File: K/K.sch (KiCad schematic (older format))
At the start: 75 parts

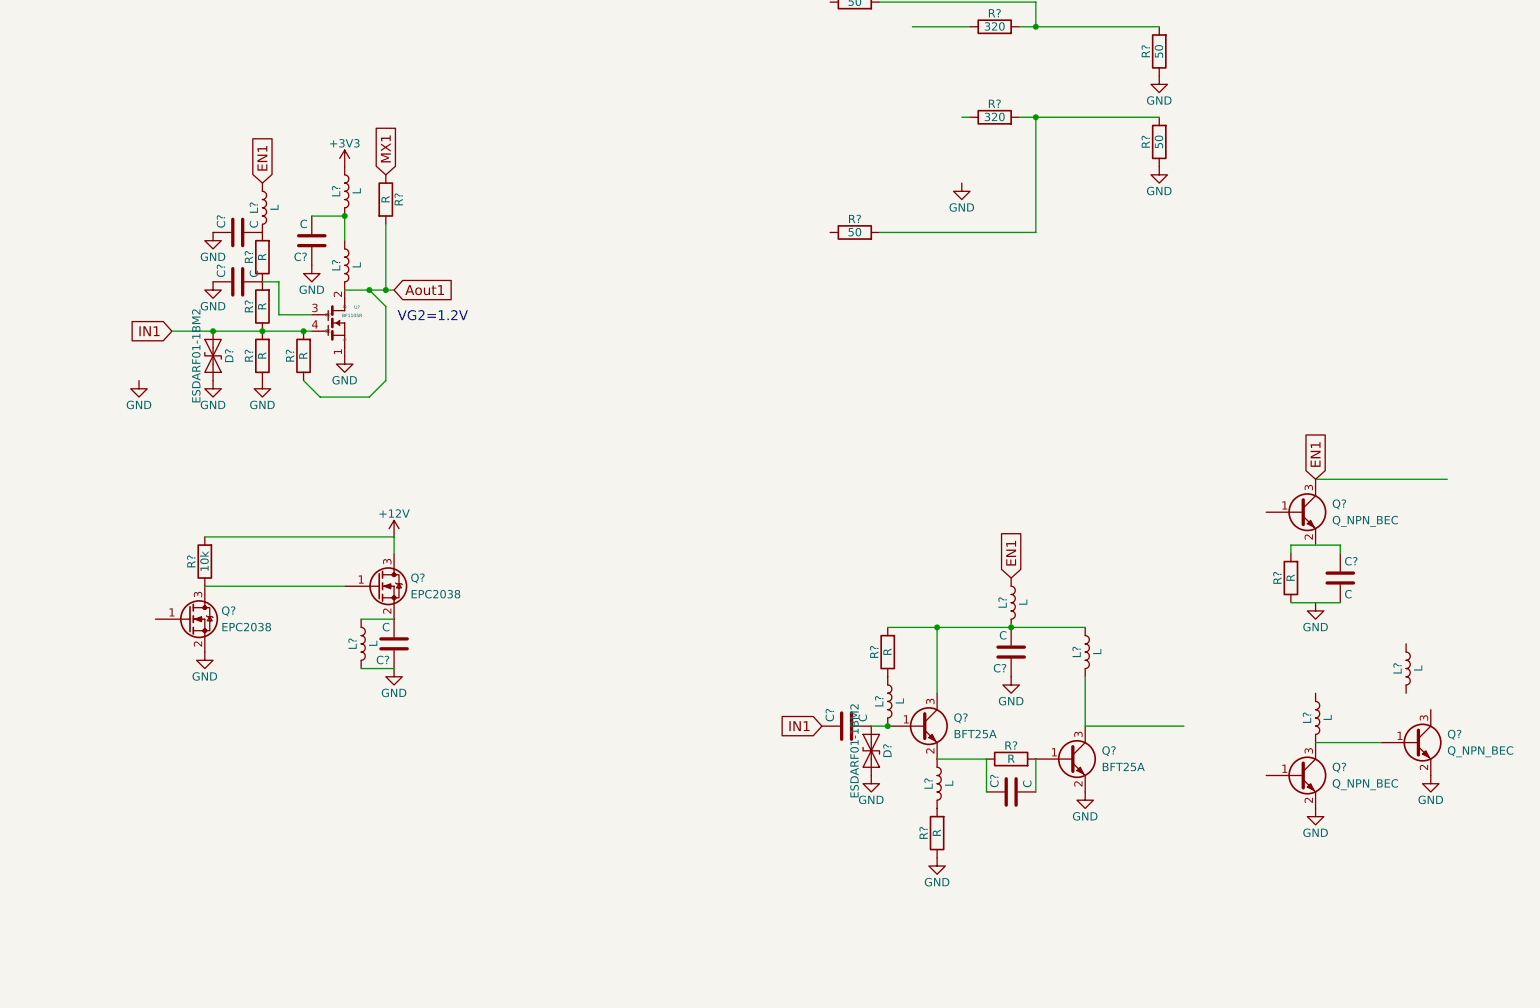
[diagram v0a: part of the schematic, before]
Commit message: f
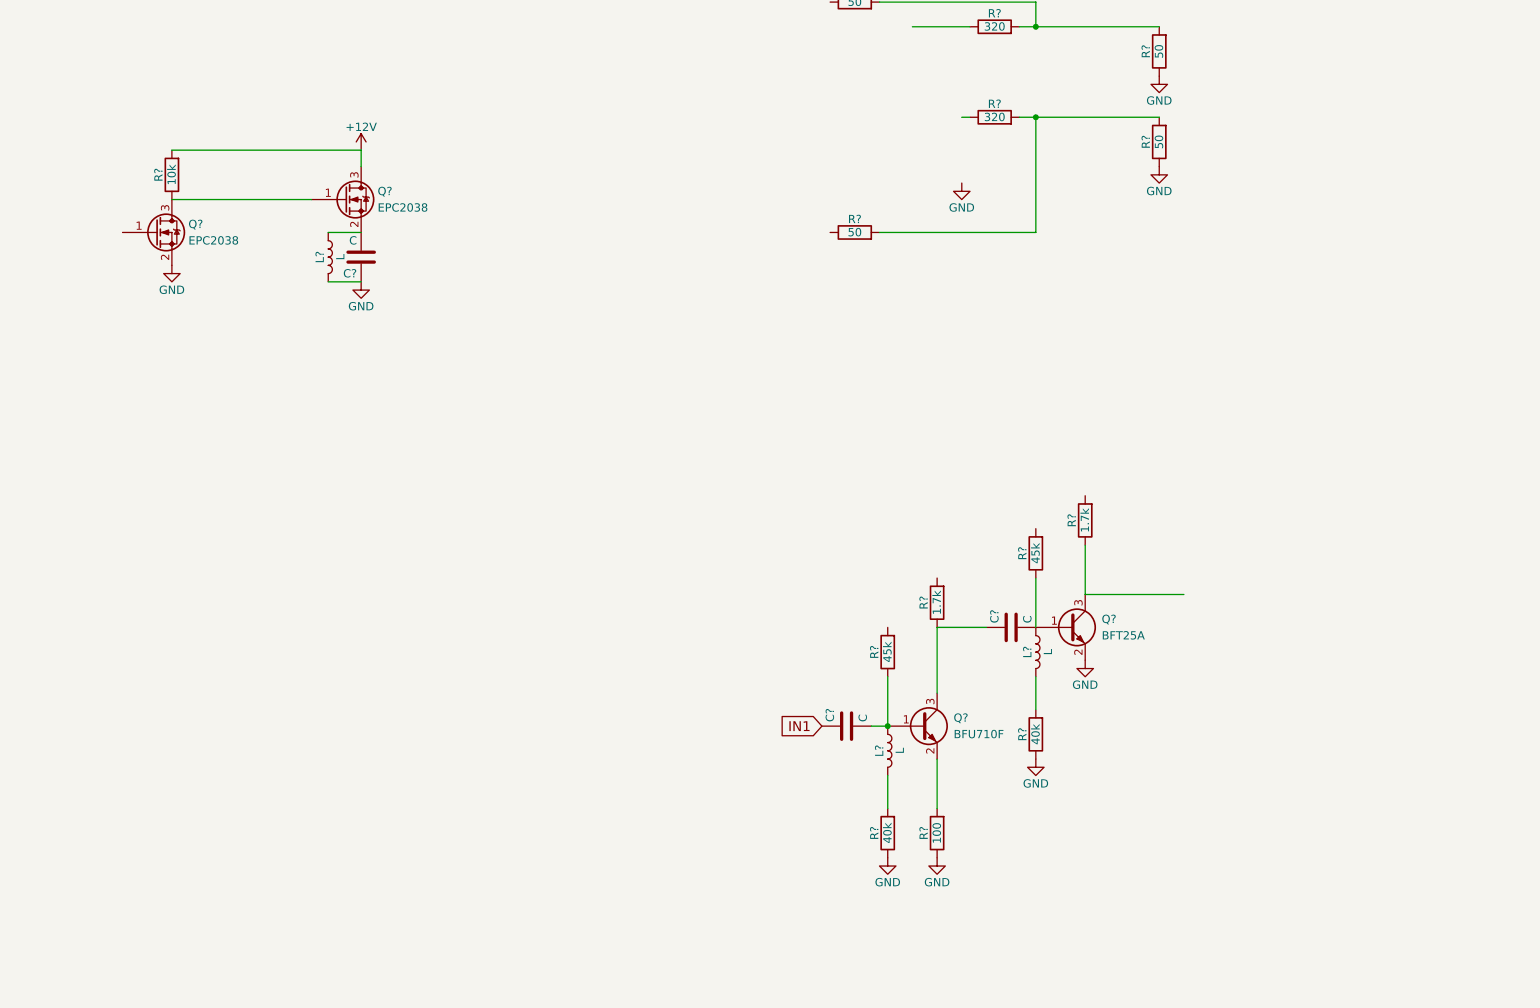
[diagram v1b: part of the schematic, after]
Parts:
- removed C? (x5): C, symbol C
- removed D? (x2): ESDARF01-1BM2, symbol D_TVS
- removed L? (x9): L, symbol L
- removed Q? (x3): Q_NPN_BEC, symbol Q_NPN_BEC
- removed R? (x7): R, symbol R
- removed U?: BF1105R, symbol BF1105R
- added L? (x2): L, symbol L
- added R? (x2): 40k, symbol R
- added R? (x2): 1.7k, symbol R
- added R?: 45k, symbol R
- Q?: value BFT25A -> BFU710F
- R?: value R -> 45k
- R?: value R -> 100
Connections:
- net labels removed: +3V3, Aout1, EN1, MX1
- wire segments 60 -> 43
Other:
- note removed: "VG2=1.2V"
- moved on the sheet: C?, L?, Q?, R?
